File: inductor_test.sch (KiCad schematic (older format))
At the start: 37 parts, among them CON1 AVR-ISP-10, J1 DC_JACK, P1 CONN_4, P2 CONN_2, P3 CONN_2, Q1 2N7000, Q2 2N7000, Q3 2N2906, Q4 2N2222A, Q5 IRLIZ24N, SW1 RotEncoder, U1 LM317LZ, U2 78L15, U3 ATTINY13A-PU, U4 74HC14

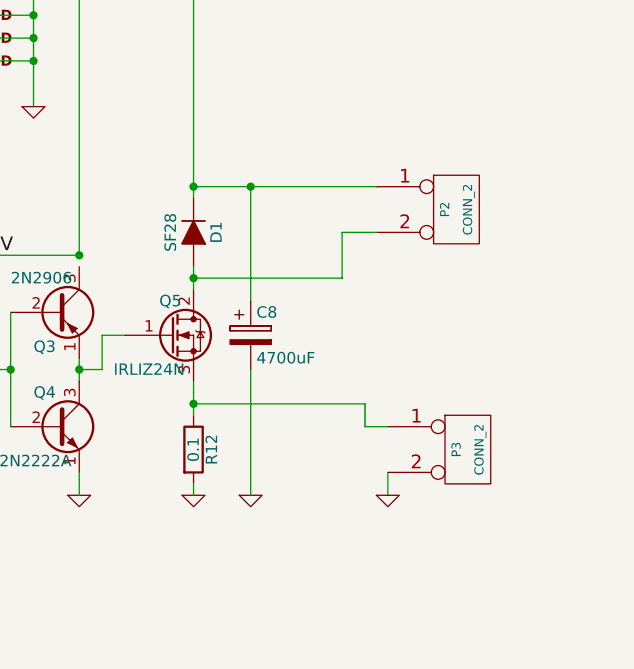
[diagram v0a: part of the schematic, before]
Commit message: ...
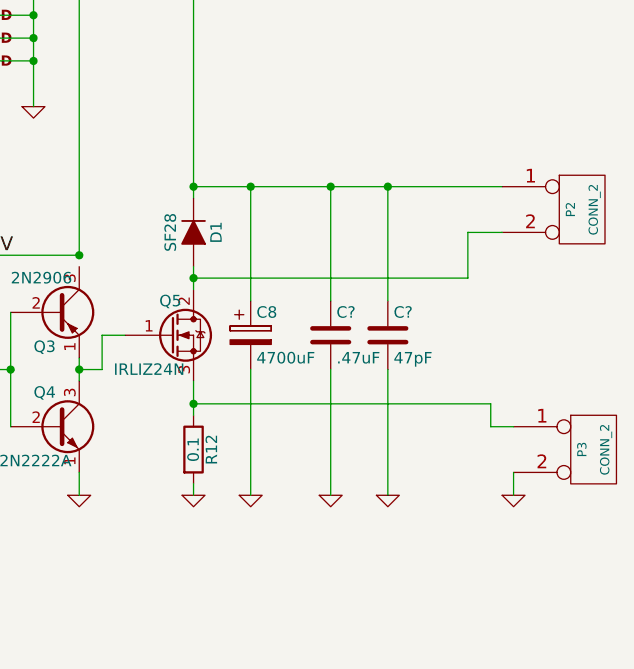
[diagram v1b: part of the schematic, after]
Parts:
- added C?: .47uF, symbol C
- added C?: 47pF, symbol C
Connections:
- net GND: now also C?.2, C?.2
- net Vin: now also C?.1, C?.1
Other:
- moved on the sheet: P2, P3
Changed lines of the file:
@@
 L CONN_2 P2
 U 1 1 595F3354
-P 9300 3850
-F 0 "P2" V 9250 3850 40  0000 C CNN
-F 1 "CONN_2" V 9350 3850 40  0000 C CNN
-F 2 "" H 9300 3850 60  0001 C CNN
-F 3 "" H 9300 3850 60  0001 C CNN
-	1    9300 3850
+P 9850 3850
+F 0 "P2" V 9800 3850 40  0000 C CNN
+F 1 "CONN_2" V 9900 3850 40  0000 C CNN
+F 2 "" H 9850 3850 60  0001 C CNN
+F 3 "" H 9850 3850 60  0001 C CNN
+	1    9850 3850
 	1    0    0    -1
 $EndComp
@@
 	8150 1000 8150 3800
 Wire Wire Line
-	8950 3950 8800 3950
-Wire Wire Line
-	8800 3950 8800 4150
-Wire Wire Line
-	8800 4150 8150 4150
+	9500 3950 9350 3950
+Wire Wire Line
+	9350 3950 9350 4150
+Wire Wire Line
+	9350 4150 8150 4150
 Connection ~ 8150 4150
 Connection ~ 8400 3750
@@
 L CONN_2 P3
 U 1 1 5964B59F
-P 9350 4900
-F 0 "P3" V 9300 4900 40  0000 C CNN
-F 1 "CONN_2" V 9400 4900 40  0000 C CNN
-F 2 "" H 9350 4900 60  0001 C CNN
-F 3 "" H 9350 4900 60  0001 C CNN
-	1    9350 4900
+P 9900 4900
+F 0 "P3" V 9850 4900 40  0000 C CNN
+F 1 "CONN_2" V 9950 4900 40  0000 C CNN
+F 2 "" H 9900 4900 60  0001 C CNN
+F 3 "" H 9900 4900 60  0001 C CNN
+	1    9900 4900
 	1    0    0    -1
 $EndComp
@@
 L GND #PWR017
 U 1 1 5964B6DA
+P 9550 5100
+F 0 "#PWR017" H 9550 5100 30  0001 C CNN
+F 1 "GND" H 9550 5030 30  0001 C CNN
+F 2 "" H 9550 5100 60  0000 C CNN
+F 3 "" H 9550 5100 60  0000 C CNN
+	1    9550 5100
+	1    0    0    -1
+$EndComp
+Wire Wire Line
+	9550 5000 9550 5100
+Wire Wire Line
+	8150 4700 9450 4700
+Wire Wire Line
+	9450 4700 9450 4800
+Wire Wire Line
+	9450 4800 9550 4800
+Connection ~ 8150 4700
+Wire Wire Line
+	6600 4050 7650 4050
+Wire Wire Line
+	8150 3750 9500 3750
+Wire Wire Line
+	1350 1000 8150 1000
+Wire Wire Line
+	3700 1400 3600 1400
+Wire Wire Line
+	4500 1400 7650 1400
+Wire Wire Line
+	7650 1400 7650 4050
+Connection ~ 3600 1000
+$Comp
+L C C?
+U 1 1 5964E1CA
+P 8750 4400
+F 0 "C?" H 8775 4500 50  0000 L CNN
+F 1 ".47uF" H 8775 4300 50  0000 L CNN
+F 2 "" H 8788 4250 50  0001 C CNN
+F 3 "" H 8750 4400 50  0001 C CNN
+	1    8750 4400
+	1    0    0    -1
+$EndComp
+$Comp
+L C C?
+U 1 1 5964E257
+P 9000 4400
+F 0 "C?" H 9025 4500 50  0000 L CNN
+F 1 "47pF" H 9025 4300 50  0000 L CNN
+F 2 "" H 9038 4250 50  0001 C CNN
+F 3 "" H 9000 4400 50  0001 C CNN
+	1    9000 4400
+	1    0    0    -1
+$EndComp
+Wire Wire Line
+	8750 4250 8750 3750
+Connection ~ 8750 3750
+Wire Wire Line
+	9000 3750 9000 4250
+Connection ~ 9000 3750
+$Comp
+L GND #PWR?
+U 1 1 5964E57B
+P 8750 5100
+F 0 "#PWR?" H 8750 5100 30  0001 C CNN
+F 1 "GND" H 8750 5030 30  0001 C CNN
+F 2 "" H 8750 5100 60  0000 C CNN
+F 3 "" H 8750 5100 60  0000 C CNN
+	1    8750 5100
+	1    0    0    -1
+$EndComp
+$Comp
+L GND #PWR?
+U 1 1 5964E5E1
 P 9000 5100
-F 0 "#PWR017" H 9000 5100 30  0001 C CNN
+F 0 "#PWR?" H 9000 5100 30  0001 C CNN
 F 1 "GND" H 9000 5030 30  0001 C CNN
 F 2 "" H 9000 5100 60  0000 C CNN
@@
 $EndComp
 Wire Wire Line
-	9000 5000 9000 5100
-Wire Wire Line
-	8150 4700 8900 4700
-Wire Wire Line
-	8900 4700 8900 4800
-Wire Wire Line
-	8900 4800 9000 4800
-Connection ~ 8150 4700
-Wire Wire Line
-	6600 4050 7650 4050
-Wire Wire Line
-	8150 3750 8950 3750
-Wire Wire Line
-	1350 1000 8150 1000
-Wire Wire Line
-	3700 1400 3600 1400
-Wire Wire Line
-	4500 1400 7650 1400
-Wire Wire Line
-	7650 1400 7650 4050
-Connection ~ 3600 1000
+	8750 4550 8750 5100
+Wire Wire Line
+	9000 4550 9000 5100
 $EndSCHEMATC
